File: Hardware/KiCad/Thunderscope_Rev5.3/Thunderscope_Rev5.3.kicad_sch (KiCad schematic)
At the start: 16 parts

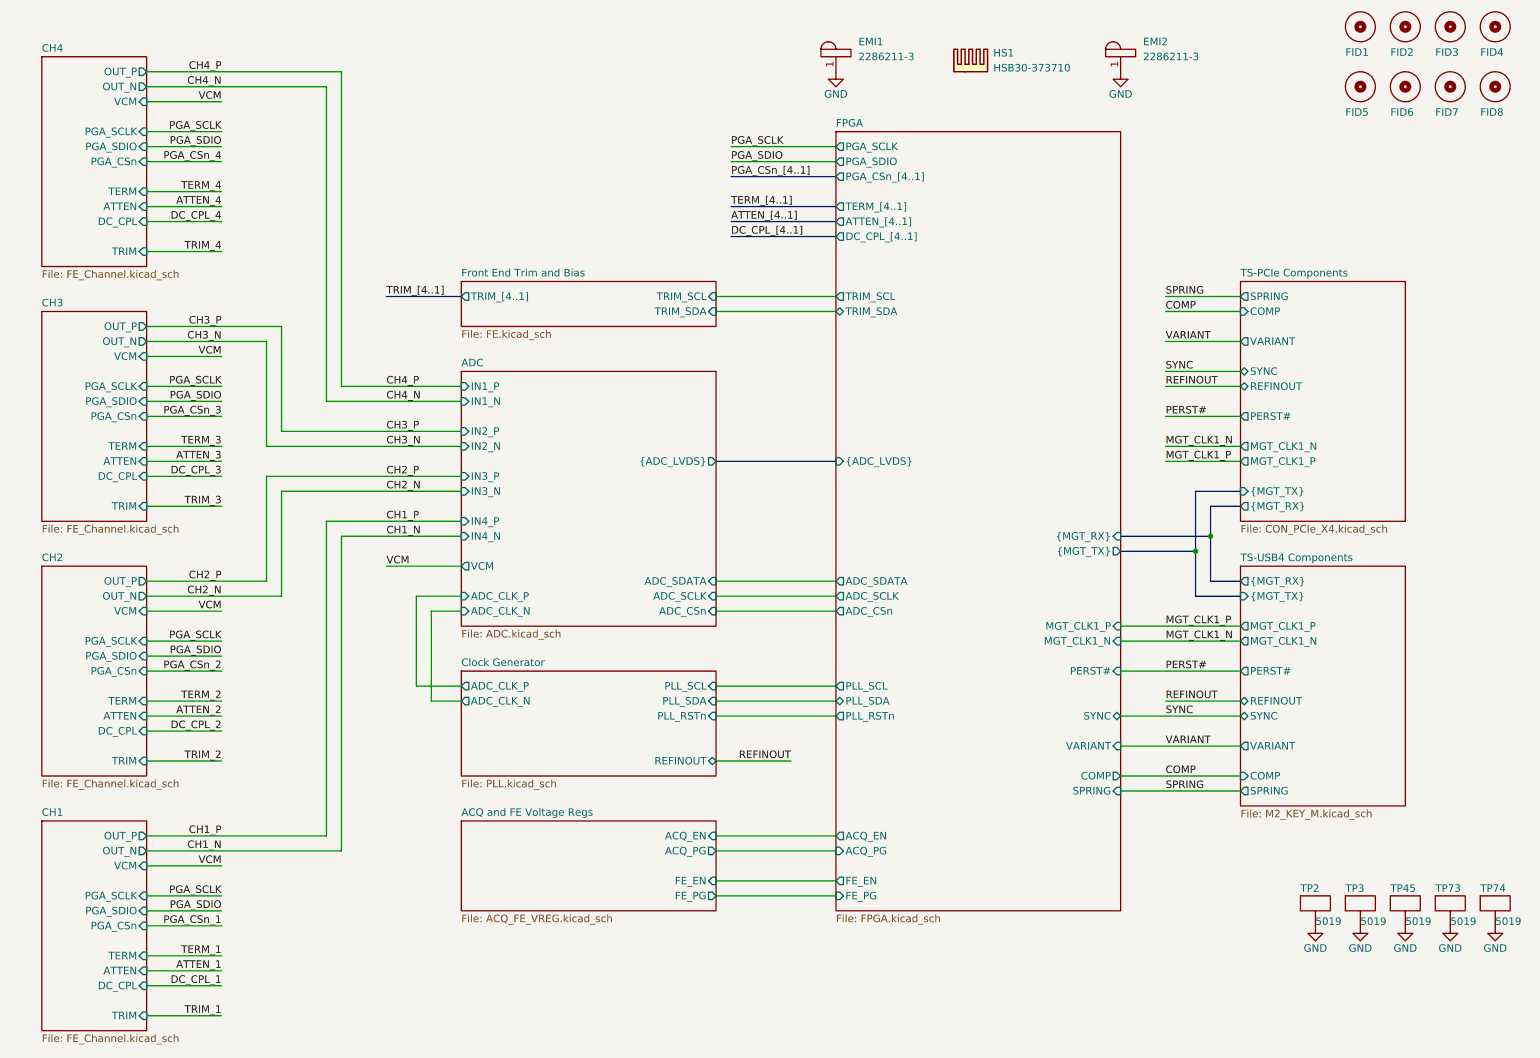
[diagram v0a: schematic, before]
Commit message: Schematic Changes for #424
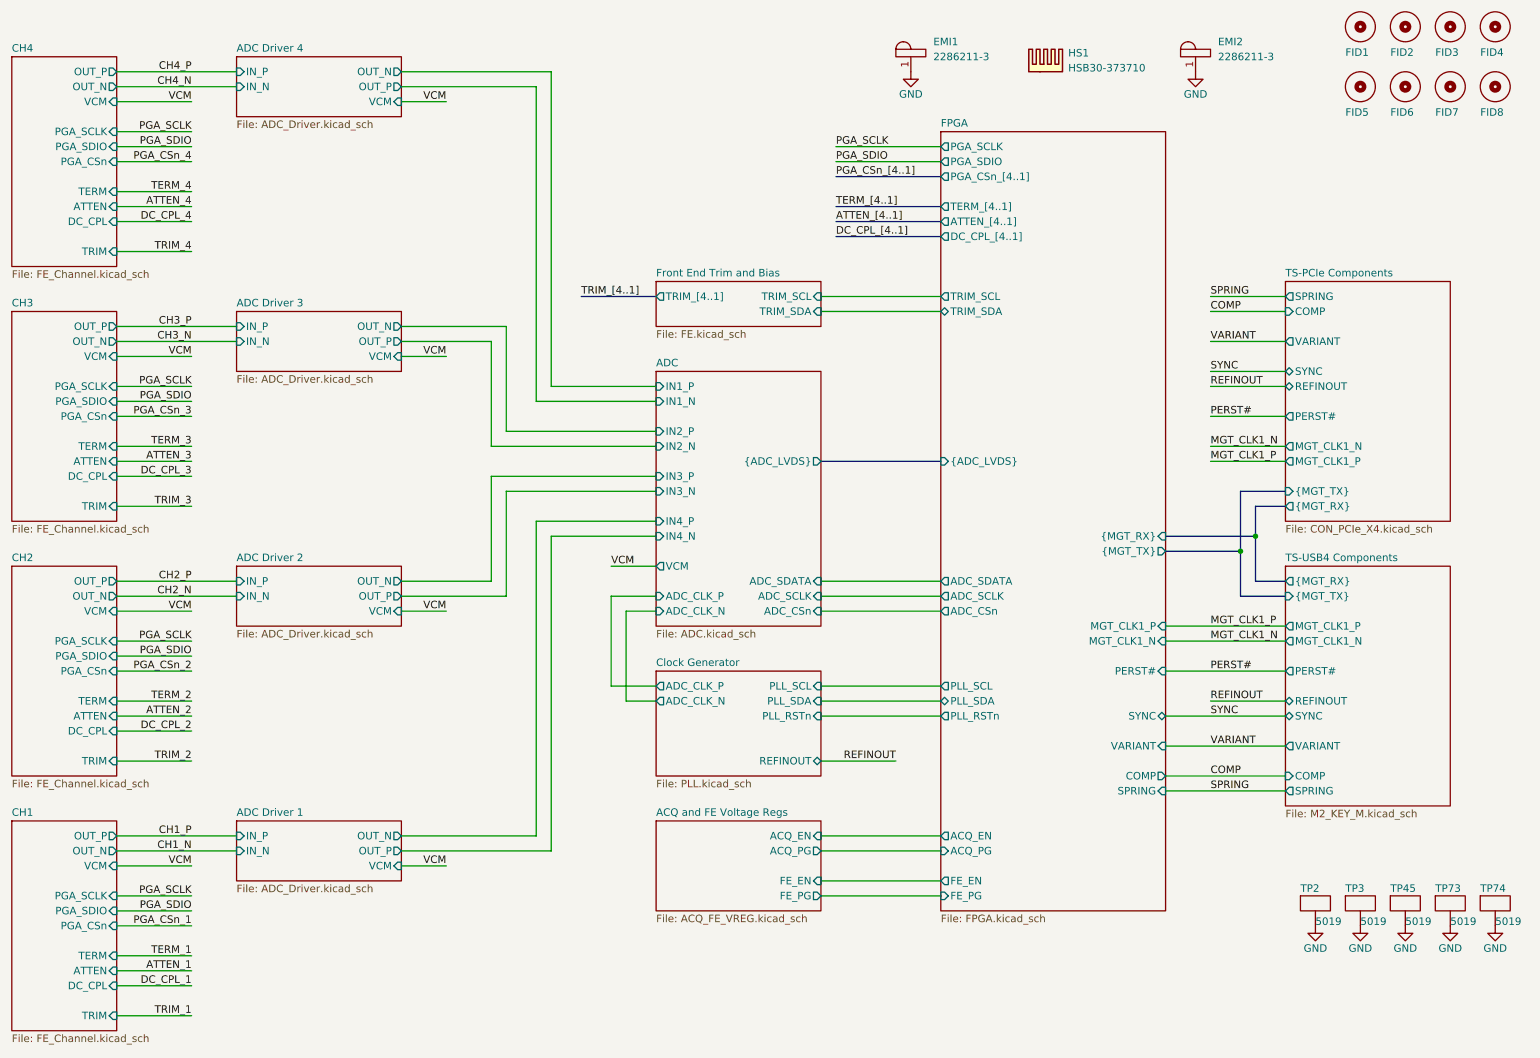
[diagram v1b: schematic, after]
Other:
- added sheet ADC Driver 1 (ADC_Driver.kicad_sch)
- added sheet ADC Driver 2 (ADC_Driver.kicad_sch)
- added sheet ADC Driver 3 (ADC_Driver.kicad_sch)
- added sheet ADC Driver 4 (ADC_Driver.kicad_sch)
- moved on the sheet: EMI1, EMI2, HS1
